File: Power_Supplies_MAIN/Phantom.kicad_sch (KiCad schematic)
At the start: 12 parts, among them IC2 LM2940IMPX-10_NOPB, IC3 XC6902NA01PR-G, J11 PINHD_1x4_Female, J13 PINHD_1x10_Female, J14 PINHD_1x10_Female

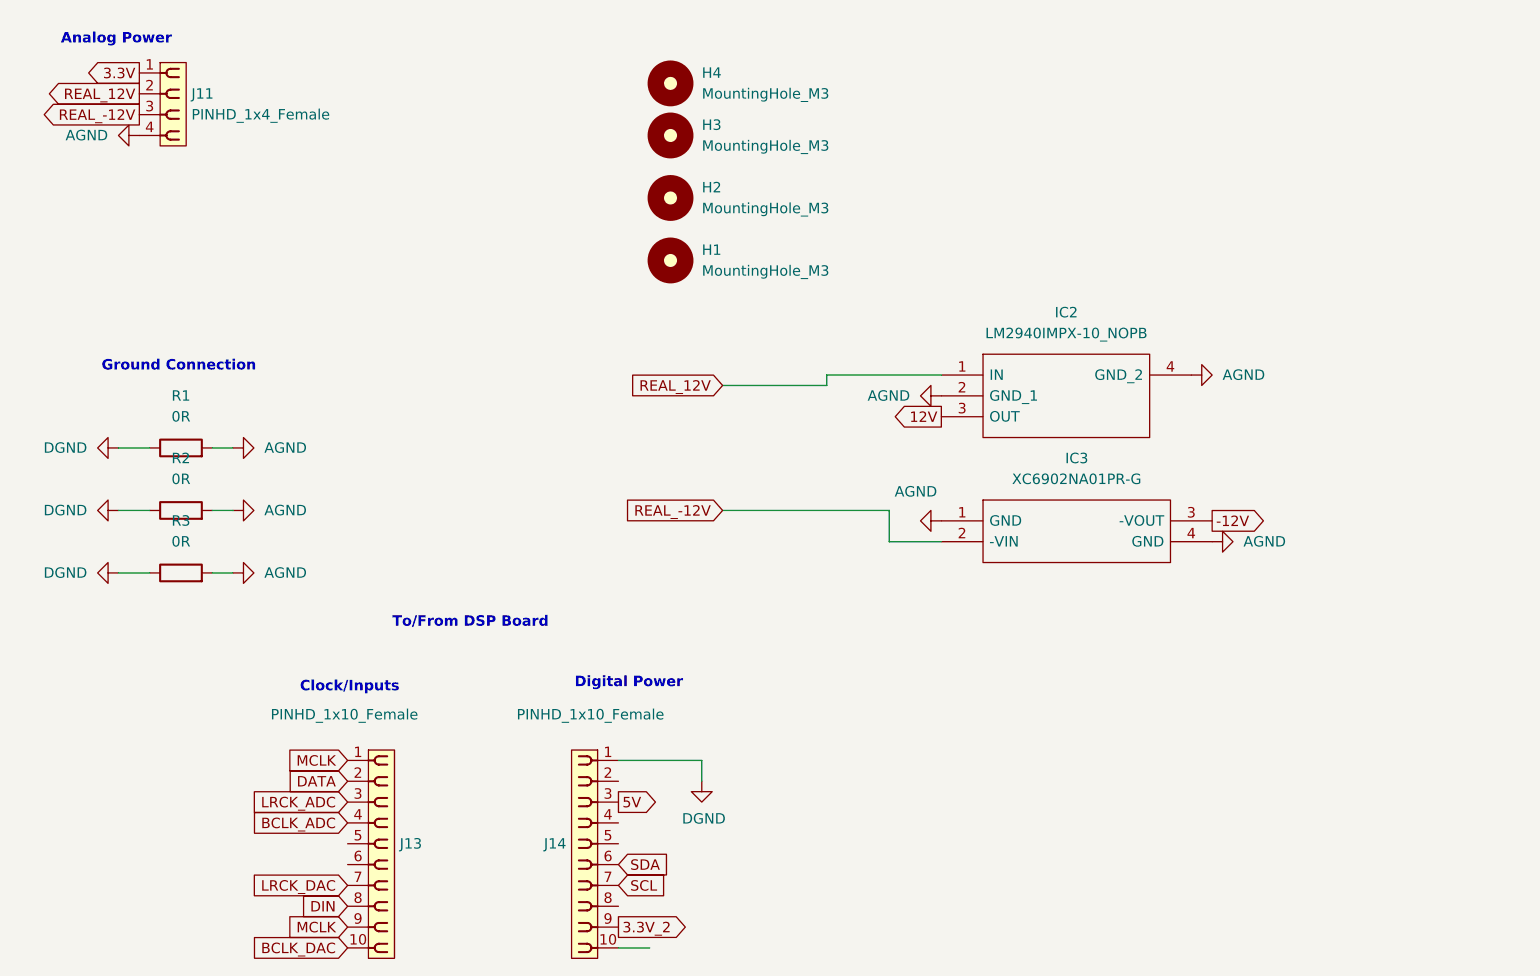
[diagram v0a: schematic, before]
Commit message: fixed a lot of stuff
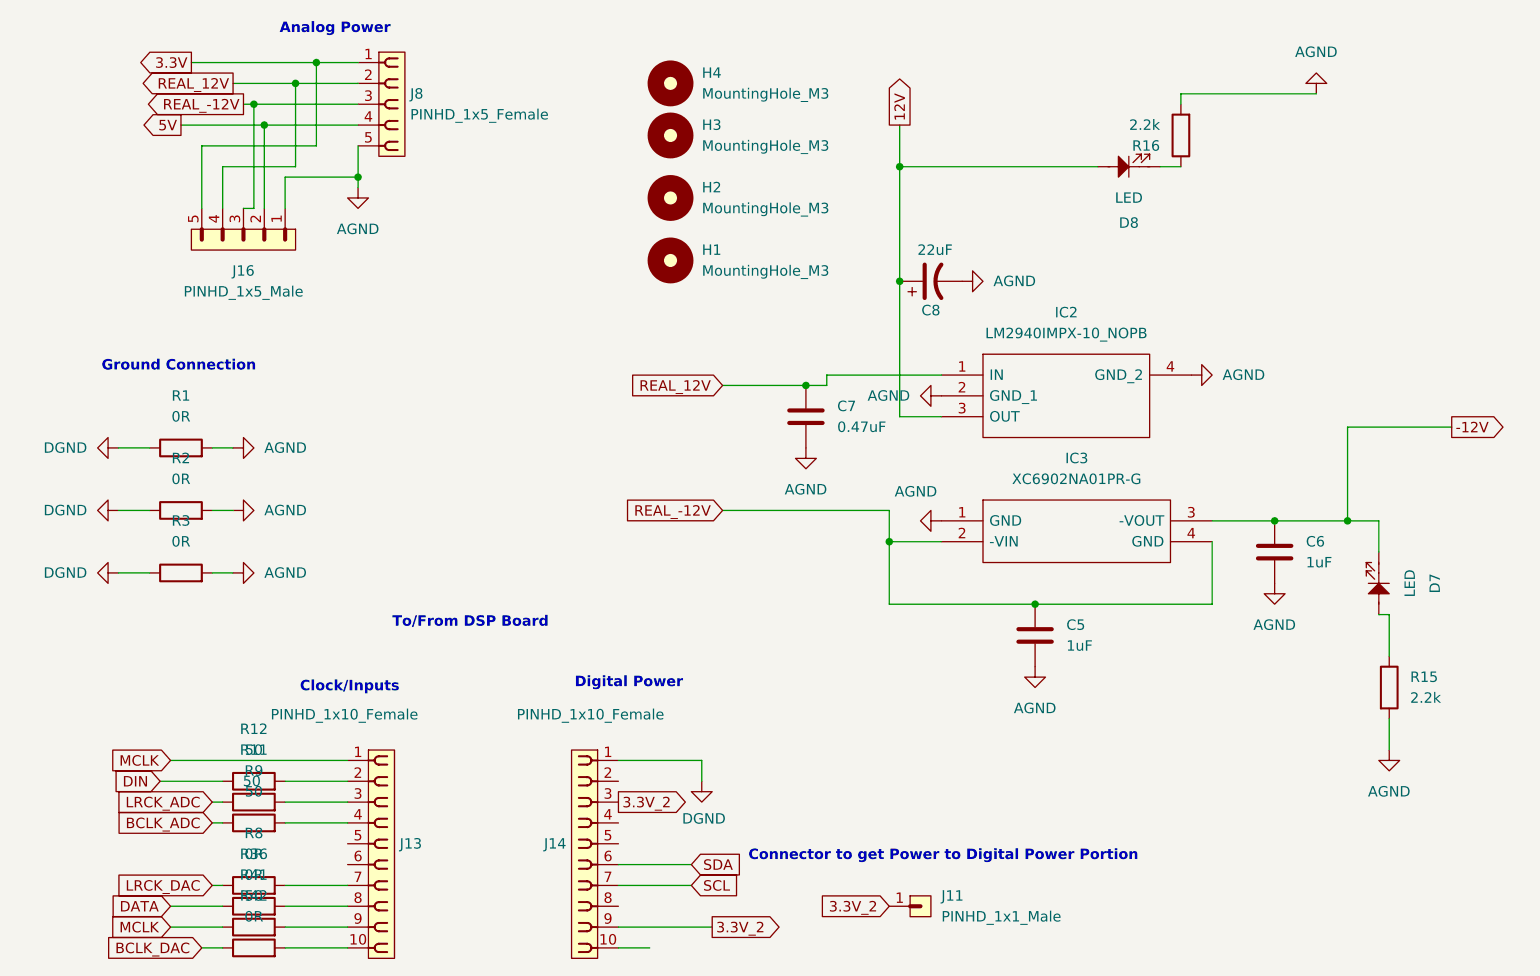
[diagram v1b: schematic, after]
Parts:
- removed J11: PINHD_1x4_Female, Connector_PinSocket_2.54mm:PinSocket_1x04_P2.54mm_Vertical, symbol PCM_SL_Pin_Headers:PINHD_1x4_Female
- added C5, C6: 1uF, PCM_Capacitor_SMD_AKL:C_0805_2012Metric, symbol PCM_Capacitor_AKL:C_0805
- added C7: 0.47uF, PCM_Capacitor_SMD_AKL:C_0805_2012Metric, symbol PCM_Capacitor_AKL:C_0805
- added C8: 22uF, Capacitor_SMD:CP_Elec_4x5.8, symbol Device:C_Polarized_US
- added D7, D8: LED, LED_SMD:LED_0402_1005Metric_Pad0.77x0.64mm_HandSolder, symbol PCM_SL_Devices:LED
- added J11: PINHD_1x1_Male, Connector_PinHeader_2.54mm:PinHeader_1x01_P2.54mm_Vertical, symbol PCM_SL_Pin_Headers:PINHD_1x1_Male
- added J16: PINHD_1x5_Male, Connector_PinHeader_2.54mm:PinHeader_1x05_P2.54mm_Vertical, symbol PCM_SL_Pin_Headers:PINHD_1x5_Male
- added J8: PINHD_1x5_Female, Connector_PinSocket_2.54mm:PinSocket_1x05_P2.54mm_Vertical, symbol PCM_SL_Pin_Headers:PINHD_1x5_Female
- added R11, R12, R41, R9: 50, Resistor_SMD:R_0805_2012Metric_Pad1.20x1.40mm_HandSolder, symbol Device:R
- added R15, R16: 2.2k, Resistor_SMD:R_0805_2012Metric, symbol Device:R
- added R36, R42, R8: 0R, Resistor_SMD:R_0805_2012Metric_Pad1.20x1.40mm_HandSolder, symbol Device:R
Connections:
- net -12V: now also C6.1, D7.1
- net 12V: now also C8.1, D8.2
- net 3.3V: now also J16.5, J8.1
- net 3.3V_2: now also J14.3, J11.1
- net 5V: now also J16.2, J8.4; no longer J14.3
- net AGND: now also C5.2, C6.2, C7.2, C8.2, J16.1, J8.5, R15.2, R16.2; no longer IC3.4 (GND)
- net BCLK_ADC: now also R9.1; no longer J13.4
- net BCLK_DAC: now also R42.1; no longer J13.10
- net DATA: now also R36.1; no longer J13.2
- net DIN: now also R12.1; no longer J13.8
- net LRCK_ADC: now also R11.1; no longer J13.3
- net LRCK_DAC: now also R8.1; no longer J13.7
- net MCLK: now also R41.1; no longer J13.9
- net REAL_-12V: now also IC3.4 (GND), C5.1, J16.3, J8.3
- net REAL_12V: now also C7.1, J16.4, J8.2
- new net: J13.9, R41.2
- new net: D8.1, R16.1
- new net: J13.2, R12.2
- new net: D7.2, R15.1
- new net: J13.7, R8.2
- new net: J13.8, R36.2
- new net: J13.10, R42.2
- new net: J13.3, R11.2
- new net: J13.4, R9.2
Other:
- note added: "Connector to get Power to Digital Power Portion"
